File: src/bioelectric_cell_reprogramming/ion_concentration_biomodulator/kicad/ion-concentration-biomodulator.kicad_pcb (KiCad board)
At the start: 4 copper layers, 165.2 x 142.7 mm, 58 parts, among them J1 532610671, J10 39-53-2045, J11 Conn_01x14_Pin, J12 Conn_01x14_Pin, J13 39-53-2045, J14 39-53-2045, J15 Conn_ARM_SWD_TagConnect_TC2030, J16 IPL1-104-01-L-D-K, J17 Conn_01x02_Pin, J18 EJ508A, J19 USB_C_Receptacle_USB2.0_14P, J2 532610671, J20 6620XX11122_66200211122, J21 IPL1-102-01-L-S-K, J3 532610671, J4 532610671, J5 S4B-PH-SM4-TB, J6 Conn_01x02_Pin, J7 6620XX11122_66200211122, J8 39-53-2045, J9 IPL1-102-01-L-S-K, Q1 NDT3055L, Q2 NDT3055L, Q3 NDT3055L, Q4 NDT3055L, Q5 NDT3055L, Q6 NDT3055L, Q7 NDT3055L, SW1 SW_Push, U1 STM32F410CBTx, U2 LM1084-5.0, U3 LM1084-3.3, U4 USBLC6-2SC6

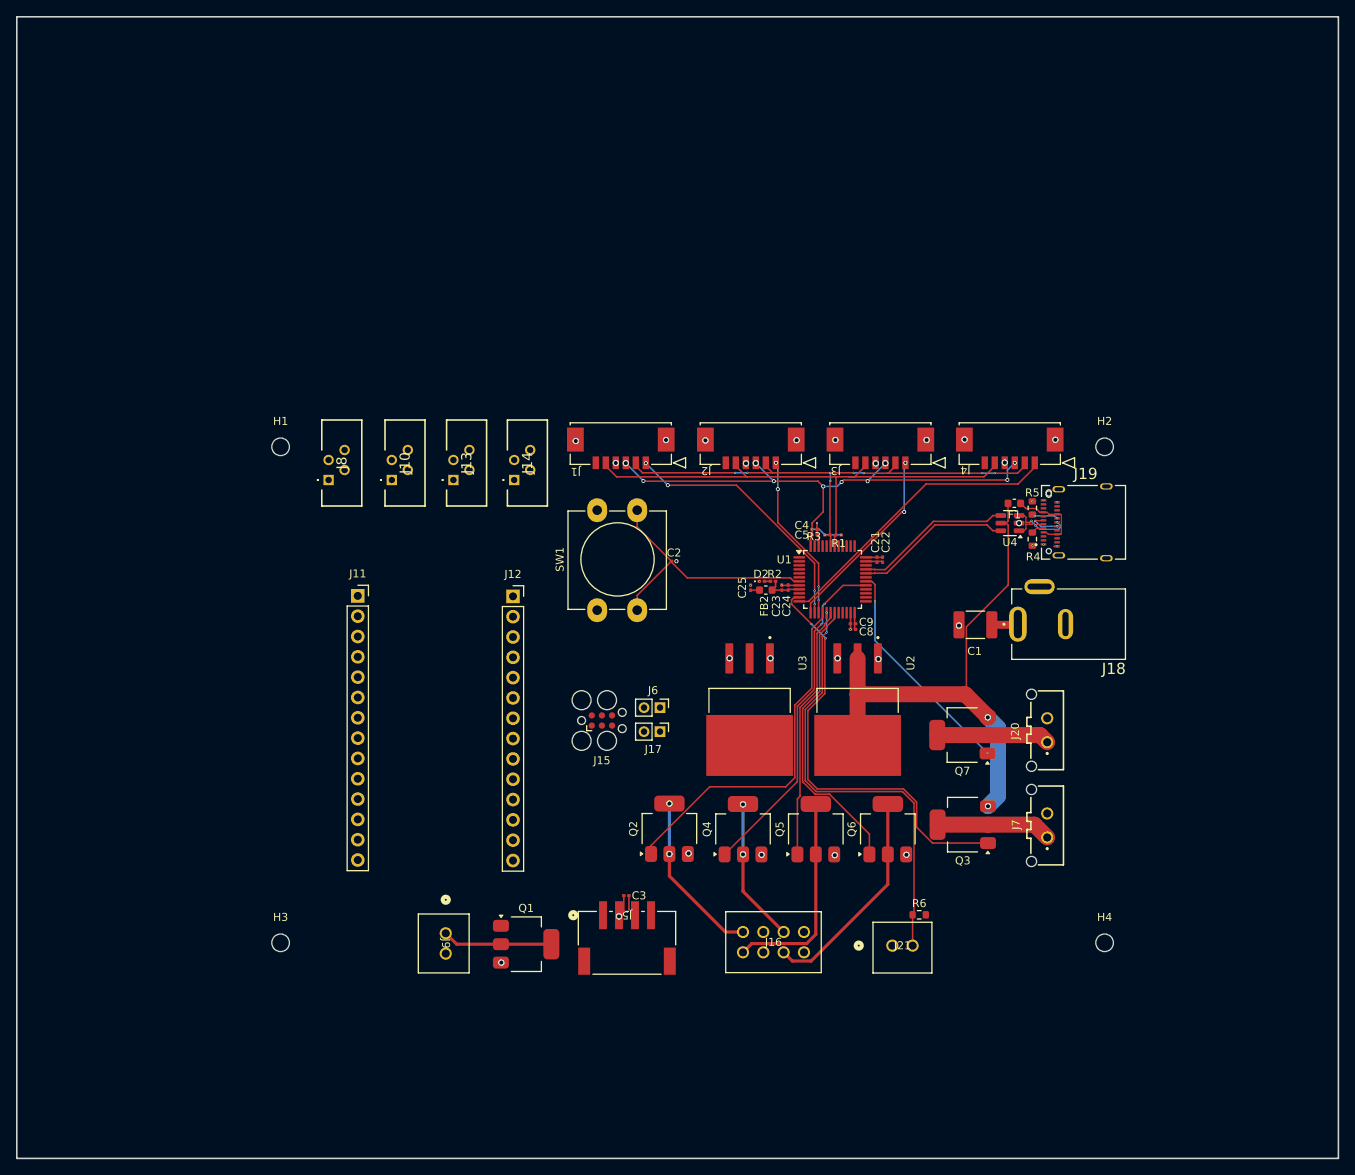
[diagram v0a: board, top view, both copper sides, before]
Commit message: refactor: re-routed icbm
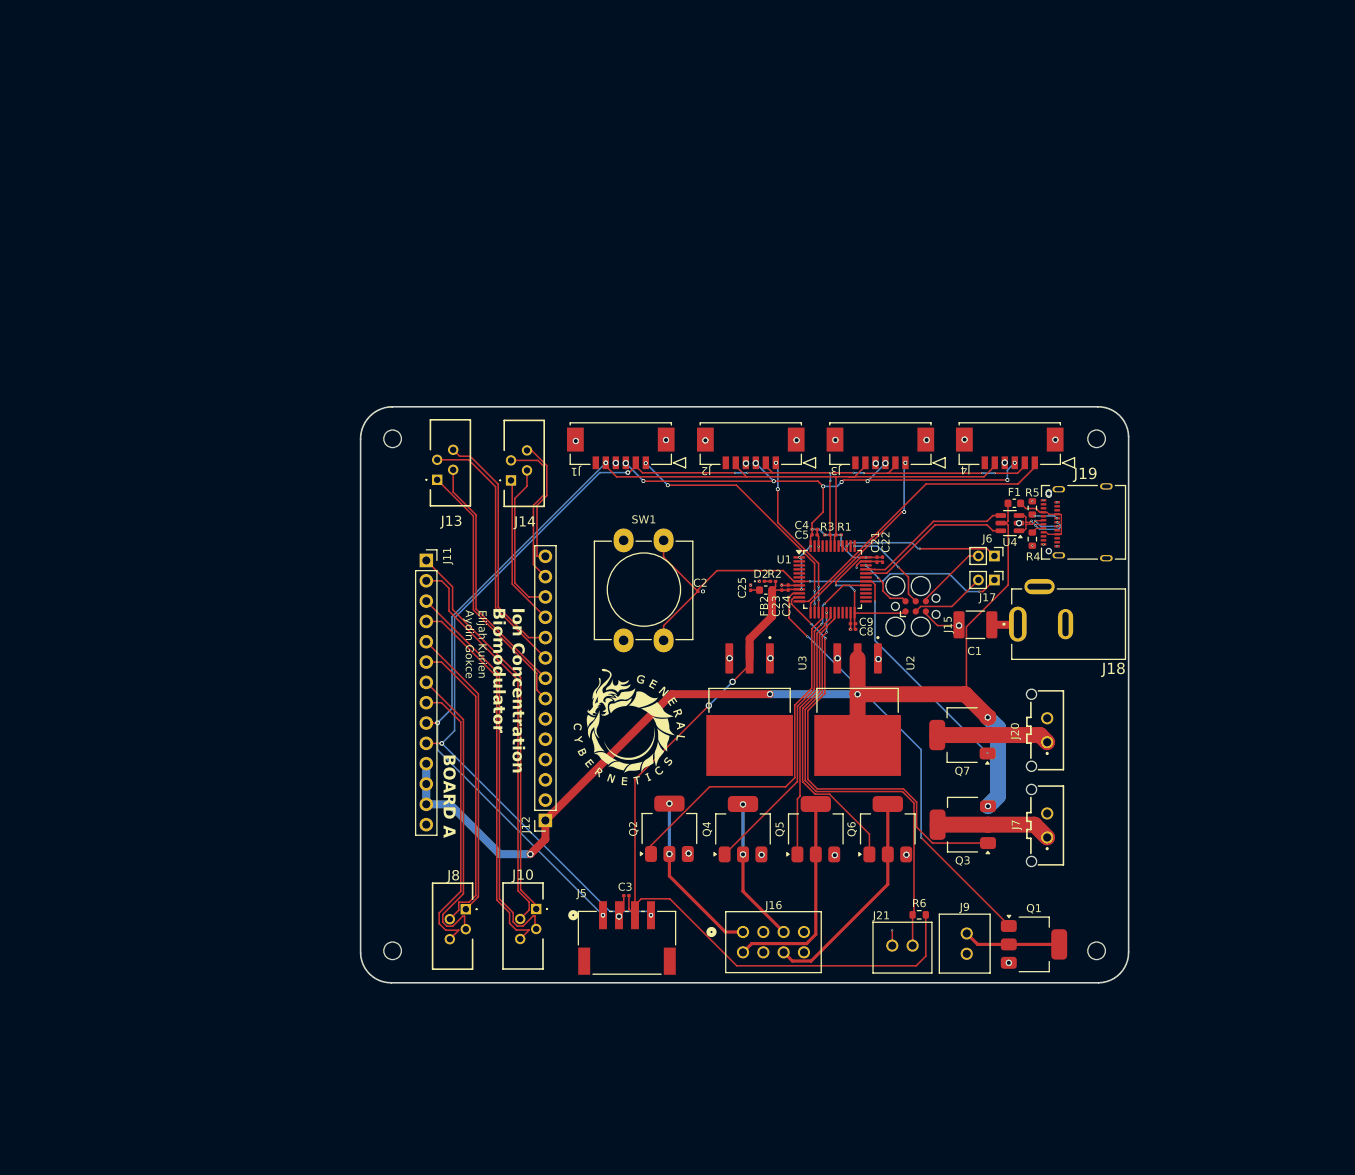
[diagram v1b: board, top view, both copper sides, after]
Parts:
- added G***: LOGO, LOGO, F.Cu at (133.0, 94.4)
- moved J9 65.1 mm to (175.2, 120.2)
- moved Q1 63.5 mm to (183.6, 121.5)
- moved J10 56.6 mm to (121.3, 117.1), turned to -90 degrees
- moved J8 56.3 mm to (112.5, 117.2), turned to -90 degrees
- moved J17 45.9 mm to (178.6, 73.0)
- moved J6 45.9 mm to (178.6, 76.0)
- moved J15 41.7 mm to (168.8, 79.3)
- moved J12 28.3 mm to (122.5, 106.1), turned to 180 degrees
- moved H1 14.0 mm to (103.4, 58.4)
- moved H3 14.0 mm to (103.4, 122.3)
- moved J11 9.64 mm to (107.6, 73.6)
- moved C2 5.01 mm to (141.9, 77.4)
- moved SW1 5.01 mm to (132.3, 83.5)
- moved J13 2.03 mm to (109.0, 63.5)
- moved H2 1.41 mm to (191.4, 58.4)
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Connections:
- U2 pad 4: (no net) -> +5V
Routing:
- net +3.3V: track 82.4 -> 205.9 mm, vias 13 -> 21
- net /I2C_SDA: track 62.7 -> 146.5 mm, vias 8 -> 11
- net /I2C_SCK: track 64.6 -> 139.9 mm, vias 0 -> 3
- net +5V: track 67.7 -> 138.9 mm, vias 2 -> 5
- net /SOLEN_OUT: track 0.00 -> 54.0 mm, vias 0 -> 2
- net /41+: track 0.00 -> 49.7 mm
- net /42-: track 0.00 -> 49.3 mm
- net /42+: track 0.00 -> 49.2 mm
- net /41-: track 0.00 -> 47.6 mm
- net /31+: track 0.00 -> 38.1 mm
- net /32+: track 0.00 -> 37.9 mm
- net /32-: track 0.00 -> 36.8 mm
- net /31-: track 0.00 -> 36.0 mm
- net /22-: track 0.00 -> 32.9 mm
- net /21+: track 0.00 -> 32.7 mm
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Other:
- board size 165.2 x 142.7 mm -> 96 x 72 mm
- board text added: "BOARD A"
- board text added: "Elijah Kurien Aydin Gokce"
- board text added: "Ion Concentration Biomodulator"
